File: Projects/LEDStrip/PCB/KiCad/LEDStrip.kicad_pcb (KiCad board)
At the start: 2 copper layers, 104.2 x 101.4 mm, 75 parts, among them J1 USB_C, J2 RGB LED, J3 LED ADDR, J4 LED MATRIX, J5 Barrel Jack, J6 SSD1306, J7 TFT, Q1 IRFML8244, Q2 IRFML8244, Q3 IRFML8244, SW1 SW_DIP_x01, SW2 SW_DIP_x01, SW3 CMD BTN, U1 MSGEQ7, U2 ESP32-S3-WROOM-1, U3 LM2596S-5, U4 AMS1117-3.3, U5 LM2596S-5, U6 MAX9814

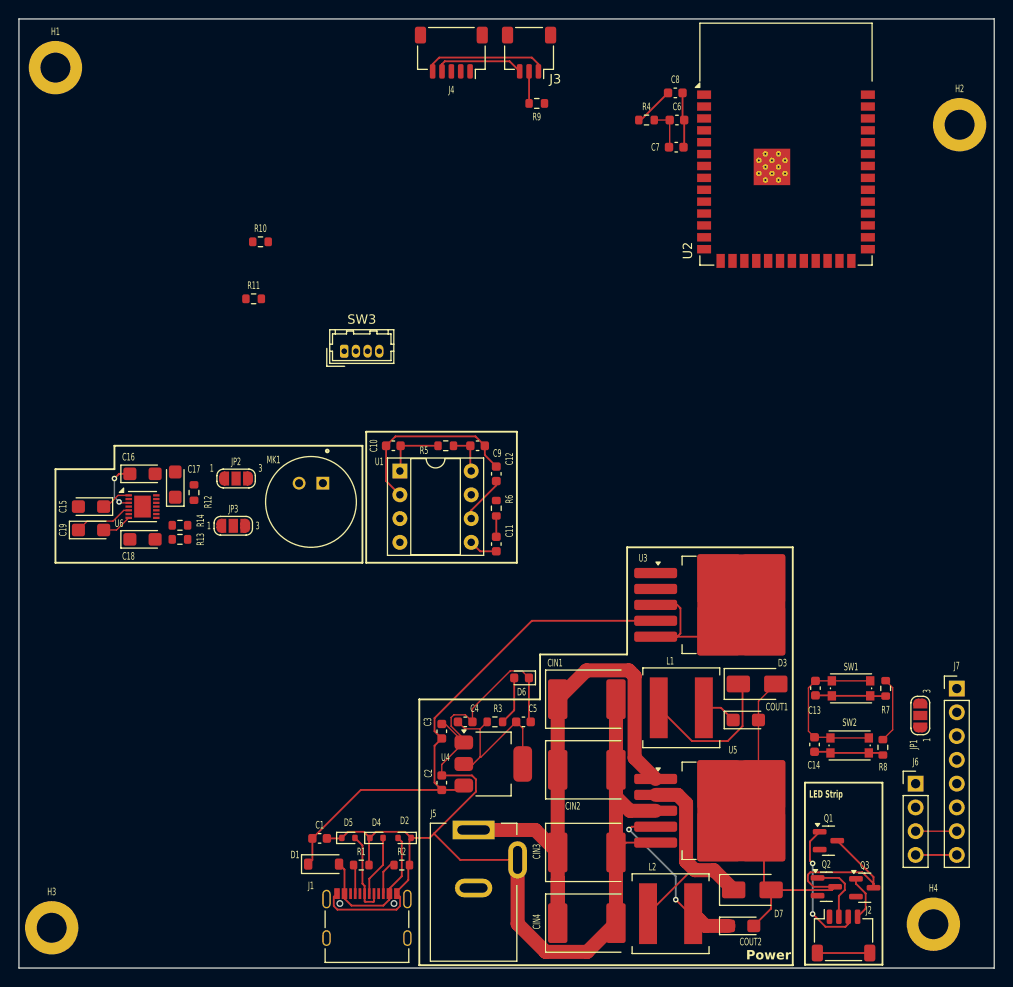
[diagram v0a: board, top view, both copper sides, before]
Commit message: pcb changes
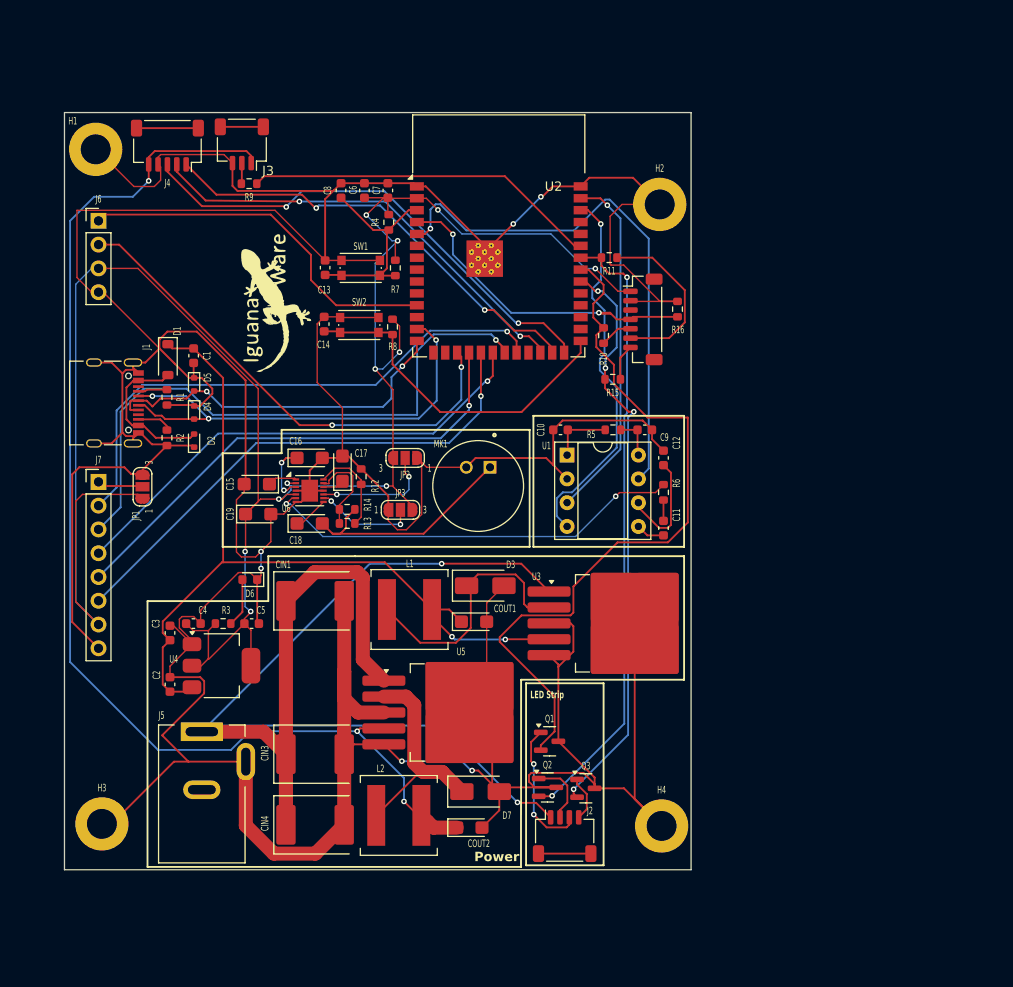
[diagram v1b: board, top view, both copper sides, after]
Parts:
- removed CIN2: 330uF, Capacitor_Tantalum_SMD:CP_EIA-7360-38_Kemet-E
- added G***: LOGO, LOGO, F.Cu at (129.9, 69.7)
- added R15: 330, Resistor_SMD:R_0603_1608Metric, F.Cu at (165.9, 77.8)
- added R16: 1k, Resistor_SMD:R_0603_1608Metric, F.Cu at (172.9, 70.3)
- R11: value 1k -> 330
- SW3: footprint Connector_Hirose:Hirose_DF13-04P-1.25DSA_1x04_P1.25mm_Vertical -> IguanaLibrary:SW_RGB_JST_SH
- moved J6 106.0 mm to (111.0, 60.9)
- moved J7 94.3 mm to (111.0, 88.8)
- moved JP1 86.6 mm to (115.7, 89.3)
- moved R8 69.0 mm to (142.4, 72.2)
- moved C13 69.0 mm to (135.2, 65.9)
- moved SW1 69.0 mm to (139.0, 65.9)
- moved SW2 69.0 mm to (138.9, 72.0)
- moved C14 69.0 mm to (135.1, 71.9)
- moved R7 69.0 mm to (142.7, 65.9)
- moved J1 61.2 mm to (112.8, 80.3), turned to -90 degrees
- moved D1 56.4 mm to (118.4, 75.7), turned to -90 degrees
- moved R1 54.1 mm to (118.3, 79.7), turned to -90 degrees
- moved C1 53.3 mm to (121.2, 75.3), turned to -90 degrees
- moved R2 52.1 mm to (118.3, 84.0), turned to -90 degrees
- moved D5 51.2 mm to (121.2, 78.3), turned to -90 degrees
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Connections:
- R10 pad 1: <NO NET> -> Net-(R10-Pad1)
- R10 pad 2: Net-(SW3-K) -> RGB_R
- R11 pad 1: <NO NET> -> Net-(R11-Pad1)
- R11 pad 2: CMD_BTN -> RGB_G
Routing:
- net <NO NET>: track 263.6 -> 608.0 mm, vias 0 -> 6
- net ESP_3V3: track 40.6 -> 233.5 mm, vias 0 -> 11
- net PER_5V: track 33.0 -> 127.0 mm, vias 2 -> 3
- net VCC_12V: track 60.3 -> 147.9 mm, vias 0 -> 2
- net RGB_R: track 0.00 -> 78.2 mm
- net RGB_G: track 0.00 -> 66.5 mm, vias 0 -> 2
- net TFT_DC: track 0.00 -> 65.6 mm, vias 0 -> 1
- net RGB_B: track 0.00 -> 62.4 mm, vias 0 -> 4
- net TFT_CS: track 0.00 -> 58.9 mm, vias 0 -> 1
- net EQ_RESET: track 0.00 -> 57.7 mm, vias 0 -> 1
- net TFT_SCLK: track 0.00 -> 55.4 mm, vias 0 -> 1
- net DISP_SCL: track 0.00 -> 53.8 mm, vias 0 -> 2
- net MAT_DIN: track 0.00 -> 53.1 mm, vias 0 -> 2
- net TFT_MOSI: track 0.00 -> 53.0 mm, vias 0 -> 1
- net TFT_RST: track 0.00 -> 52.3 mm, vias 0 -> 1
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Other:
- board size 104.2 x 101.4 mm -> 67 x 80.9 mm
